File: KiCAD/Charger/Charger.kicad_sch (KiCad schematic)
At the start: 13 parts, among them J1 Screw_Terminal_01x02, J100 Conn_01x09_Socket, J2 Conn_01x04_Socket, J3 Conn_01x04_Socket, J5 Conn_01x05_Pin, U1 ESP32-S3-DevKitC, U2 CR2013-MI2120, U3 SN65HVD230

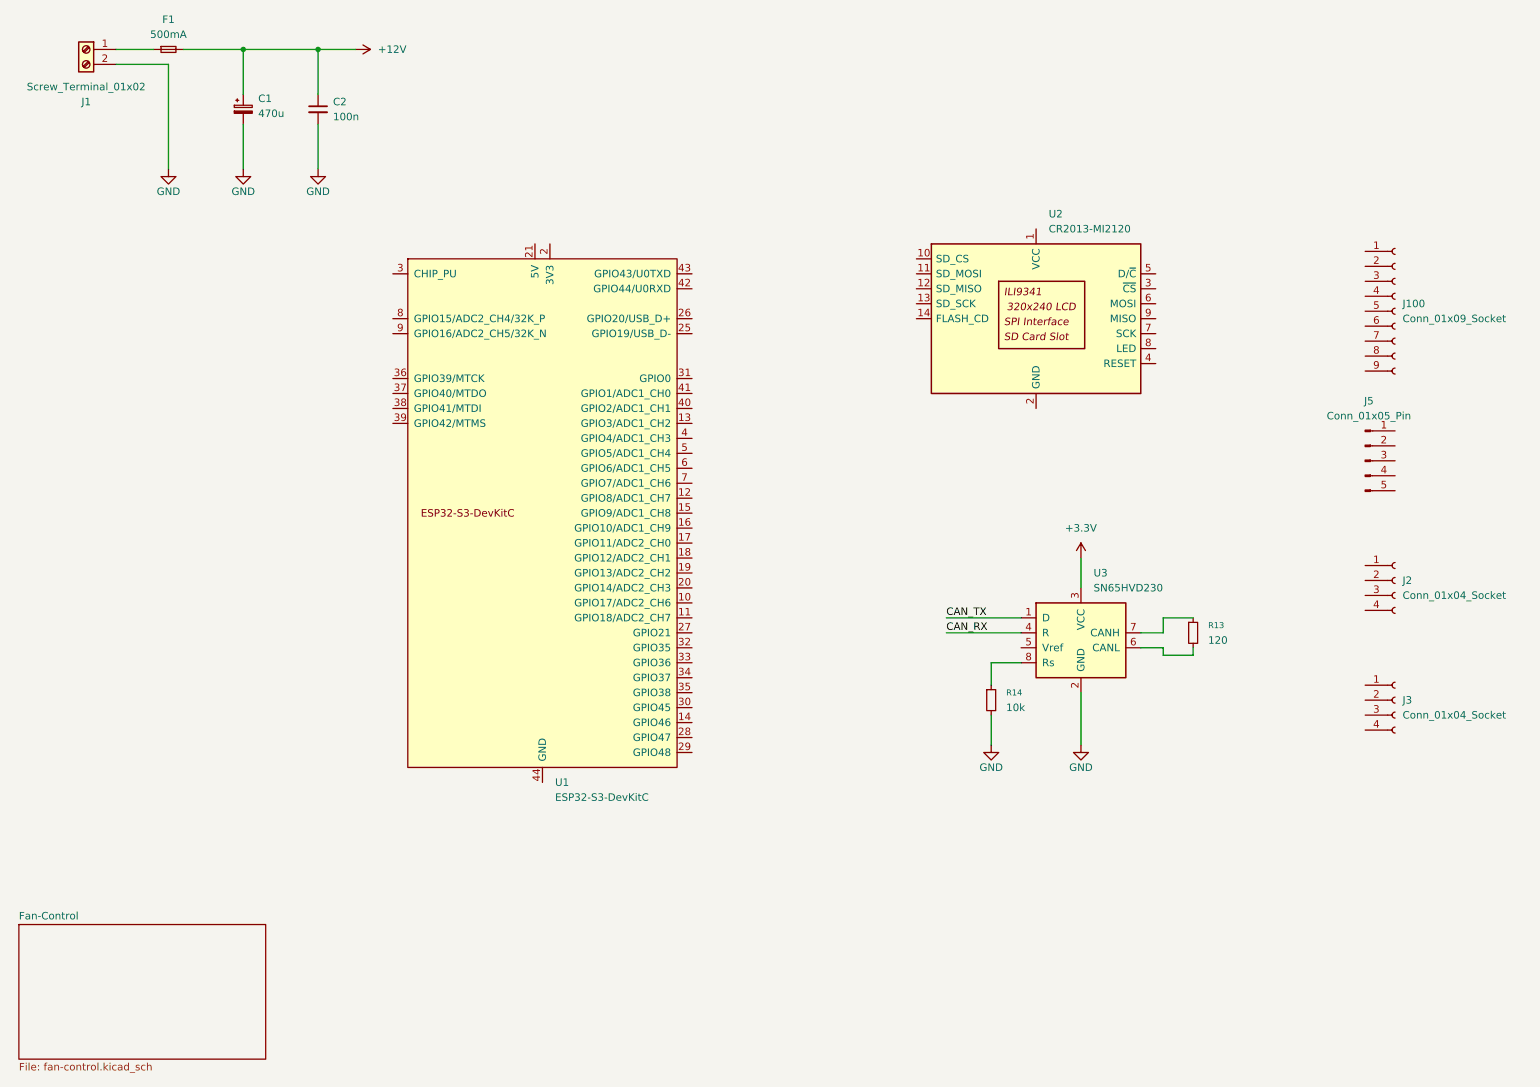
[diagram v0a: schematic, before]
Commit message: Update shematics
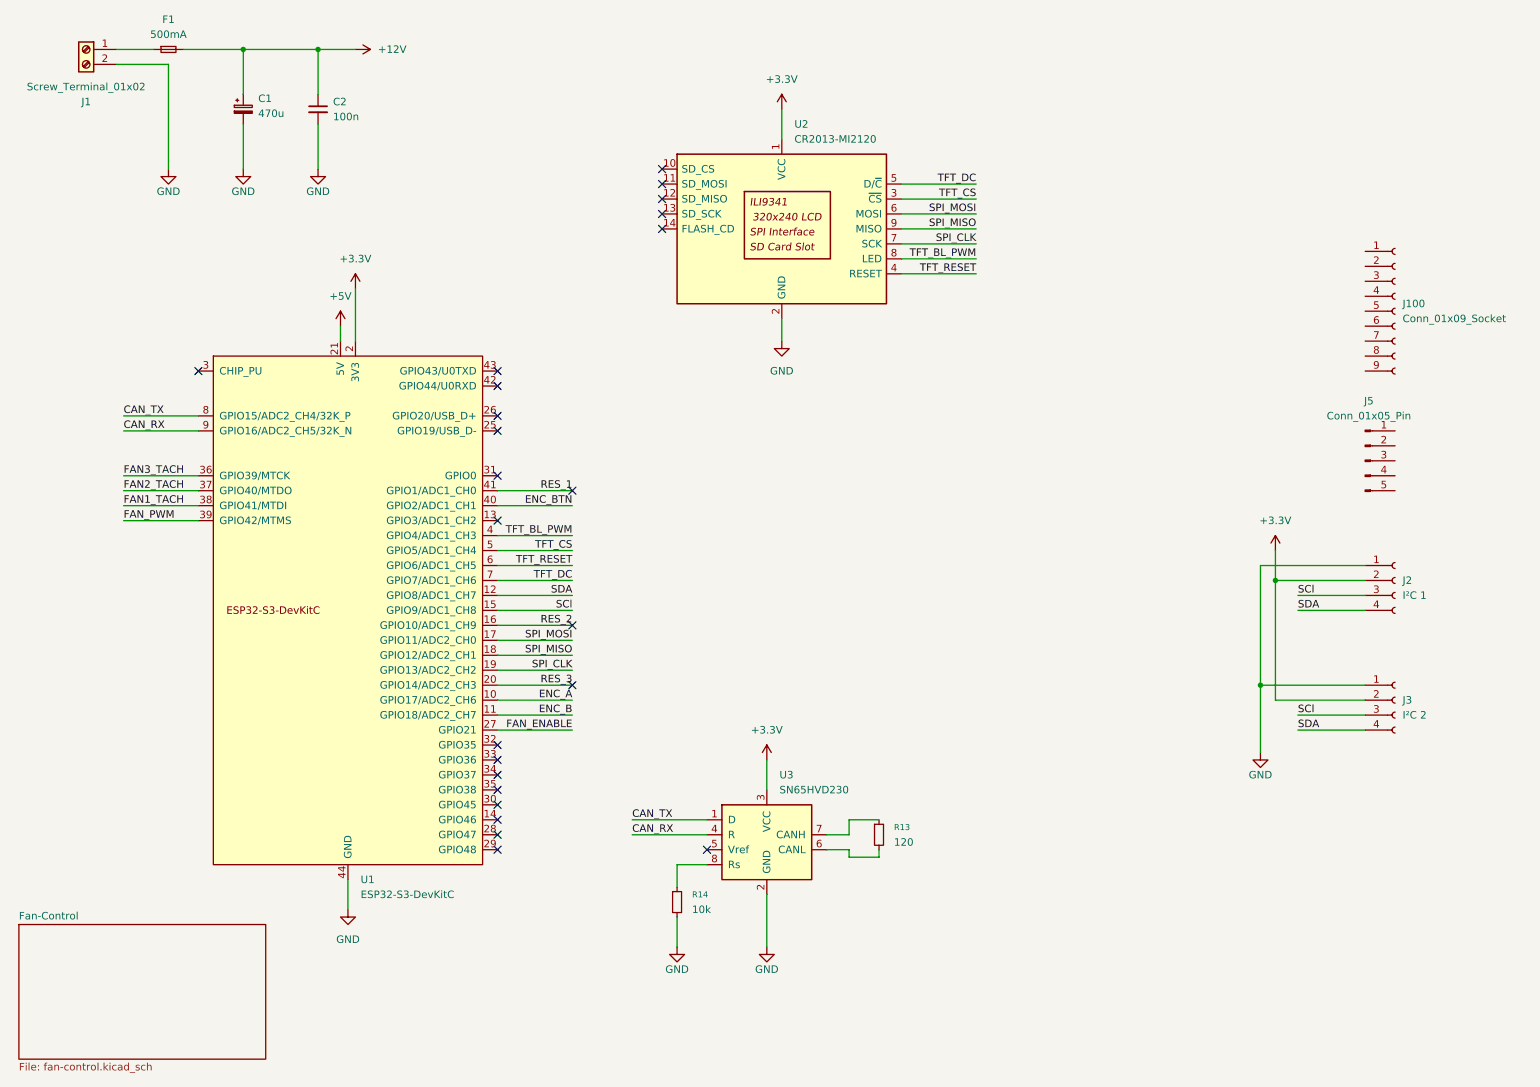
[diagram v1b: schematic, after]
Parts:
- J2: value Conn_01x04_Socket -> I²C 1
- J3: value Conn_01x04_Socket -> I²C 2
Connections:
- net +3.3V: now also J2.2 (Pin_2), J3.2 (Pin_2), U1.1 (3V3), U1.2 (3V3), U2.1 (VCC)
- net CAN_RX: now also U1.9 (GPIO16/ADC2_CH5/32K_N)
- net CAN_TX: now also U1.8 (GPIO15/ADC2_CH4/32K_P)
- net GND: now also J2.1 (Pin_1), J3.1 (Pin_1), U1.22 (GND), U1.23 (GND), U1.24 (GND), U1.44 (GND), U2.2 (GND)
- net SCl: now reaches J3.3 (Pin_3)
- net SCl: now also J2.3 (Pin_3), U1.15 (GPIO9/ADC1_CH8)
- net SDA: now reaches J3.4 (Pin_4)
- net SDA: now also J2.4 (Pin_4), U1.12 (GPIO8/ADC1_CH7)
- net TFT_CS: now reaches U2.3 (~{CS})
- net TFT_CS: now also U1.5 (GPIO5/ADC1_CH4)
- net TFT_RESET: now reaches U2.4 (RESET)
- net TFT_RESET: now also U1.6 (GPIO6/ADC1_CH5)
- net TFT_DC: now reaches U2.5 (D/~{C})
- net TFT_DC: now also U1.7 (GPIO7/ADC1_CH6)
- net SPI_MOSI: now reaches U2.6 (MOSI)
- net SPI_MOSI: now also U1.17 (GPIO11/ADC2_CH0)
- net SPI_CLK: now reaches U2.7 (SCK)
- net SPI_CLK: now also U1.19 (GPIO13/ADC2_CH2)
- net TFT_BL_PWM: now reaches U2.8 (LED)
- net TFT_BL_PWM: now also U1.4 (GPIO4/ADC1_CH3)
- net SPI_MISO: now reaches U2.9 (MISO)
- net SPI_MISO: now also U1.18 (GPIO12/ADC2_CH1)
- net ENC_A: now reaches U1.10 (GPIO17/ADC2_CH6)
- net ENC_B: now reaches U1.11 (GPIO18/ADC2_CH7)
- net RES_2: now reaches U1.16 (GPIO10/ADC1_CH9)
- net RES_3: now reaches U1.20 (GPIO14/ADC2_CH3)
- net +5V: now reaches U1.21 (5V)
- net FAN_ENABLE: now reaches U1.27 (GPIO21)
- net FAN3_TACH: now reaches U1.36 (GPIO39/MTCK)
- net FAN2_TACH: now reaches U1.37 (GPIO40/MTDO)
- net FAN1_TACH: now reaches U1.38 (GPIO41/MTDI)
- net FAN_PWM: now reaches U1.39 (GPIO42/MTMS)
- net ENC_BTN: now reaches U1.40 (GPIO2/ADC1_CH1)
- net RES_1: now reaches U1.41 (GPIO1/ADC1_CH0)
- no-connect marks 0 -> 24
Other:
- moved on the sheet: R13, R14, U1, U2, U3
